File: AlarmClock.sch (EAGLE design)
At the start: 22 parts, among them IC1 LD1117AS33TR, T1 BC817-25LT1SMD

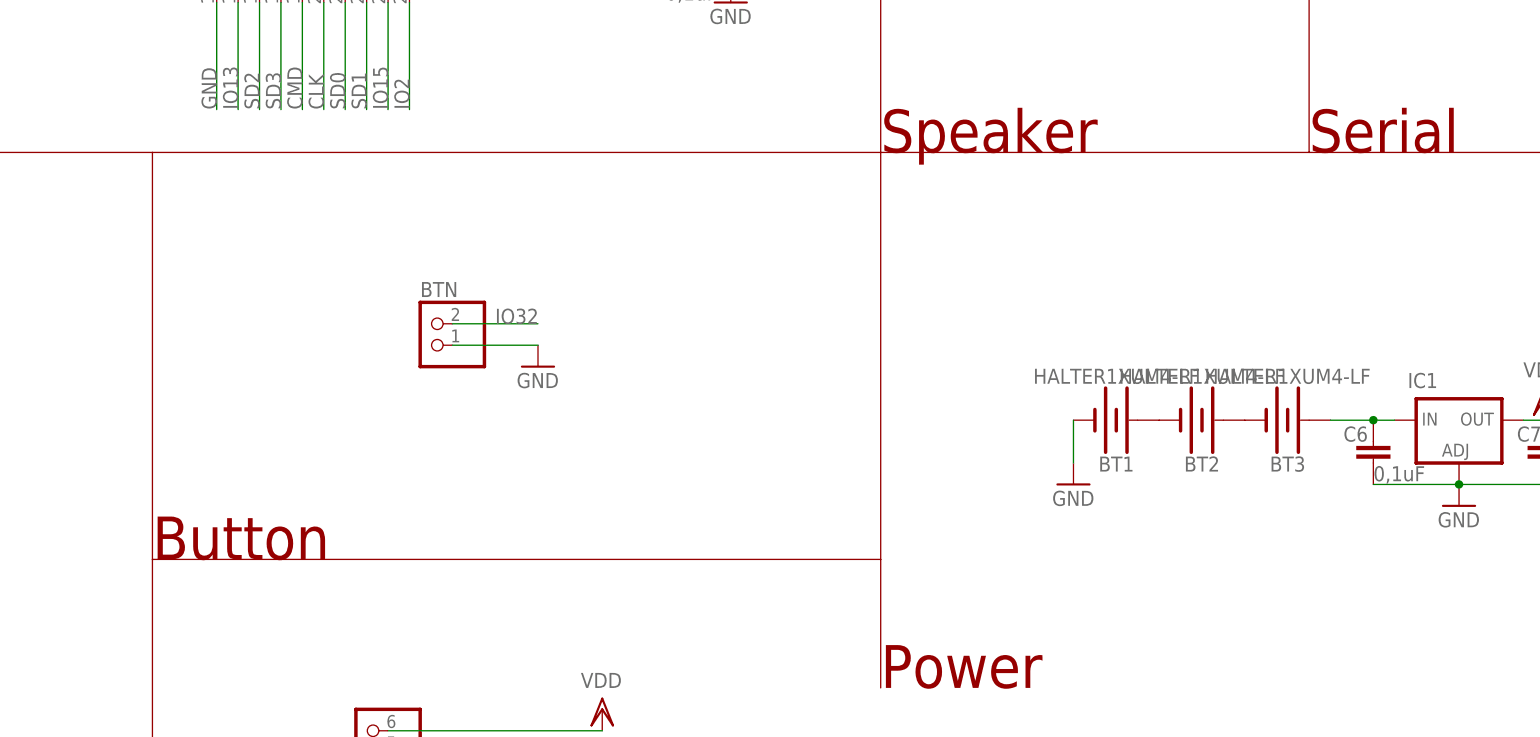
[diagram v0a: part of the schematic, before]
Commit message: Add files via upload
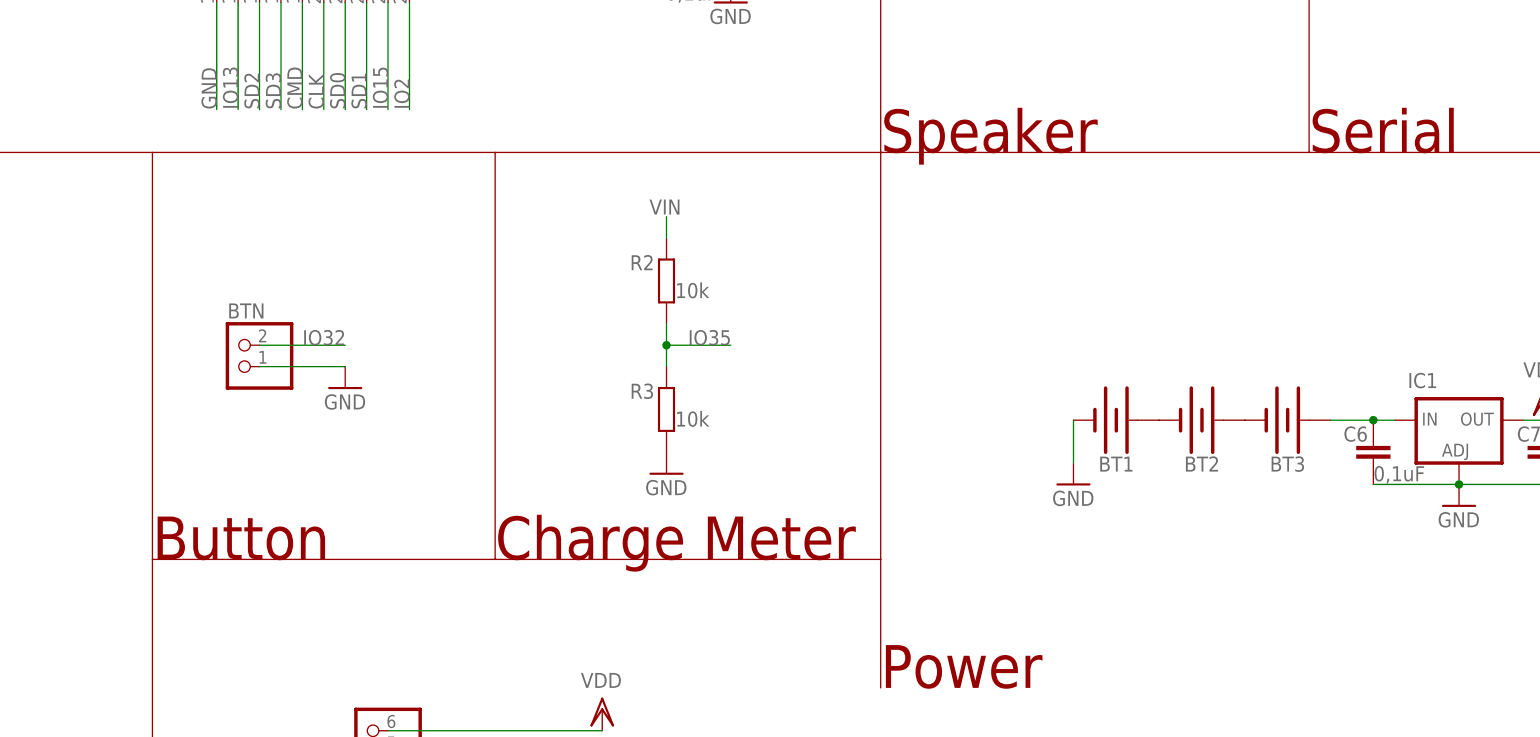
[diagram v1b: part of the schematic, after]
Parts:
- added R2, R3: 10k, rcl:R-EU_R1206
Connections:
- net GND: now also R3.1
- net IO35: now also R2.1, R3.2
- net VIN: now also R2.2
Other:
- note added: "Charge Meter"
- moved on the sheet: BTN
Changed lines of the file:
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@@
 <part name="GND9" library="supply1" library_urn="urn:adsk.eagle:library:371" deviceset="GND" device=""/>
 <part name="RST" library="rcl" library_urn="urn:adsk.eagle:library:334" deviceset="R-EU_" device="R1206" package3d_urn="urn:adsk.eagle:package:23540/2"/>
+<part name="R2" library="rcl" library_urn="urn:adsk.eagle:library:334" deviceset="R-EU_" device="R1206" package3d_urn="urn:adsk.eagle:package:23540/2" value="10k"/>
+<part name="R3" library="rcl" library_urn="urn:adsk.eagle:library:334" deviceset="R-EU_" device="R1206" package3d_urn="urn:adsk.eagle:package:23540/2" value="10k"/>
+<part name="GND10" library="supply1" library_urn="urn:adsk.eagle:library:371" deviceset="GND" device=""/>
 </parts>
 <sheets>
@@
 <text x="162.56" y="35.56" size="5.08" layer="94">Power</text>
 <text x="253.492" y="7.112" size="2.54" layer="94">1.0</text>
-<wire x1="162.56" y1="99.06" x2="76.2" y2="99.06" width="0.1524" layer="94"/>
+<wire x1="162.56" y1="99.06" x2="116.84" y2="99.06" width="0.1524" layer="94"/>
+<wire x1="116.84" y1="99.06" x2="76.2" y2="99.06" width="0.1524" layer="94"/>
 <wire x1="76.2" y1="99.06" x2="0" y2="99.06" width="0.1524" layer="94"/>
 <wire x1="162.56" y1="99.06" x2="162.56" y2="180.34" width="0.1524" layer="94"/>
@@
 <wire x1="76.2" y1="0" x2="76.2" y2="50.8" width="0.1524" layer="94"/>
 <wire x1="76.2" y1="50.8" x2="76.2" y2="99.06" width="0.1524" layer="94"/>
-<wire x1="76.2" y1="50.8" x2="162.56" y2="50.8" width="0.1524" layer="94"/>
+<wire x1="76.2" y1="50.8" x2="116.84" y2="50.8" width="0.1524" layer="94"/>
 <text x="0" y="0" size="5.08" layer="94">LCD</text>
 <text x="76.2" y="0" size="5.08" layer="94">Sensor</text>
@@
 <text x="213.36" y="99.06" size="5.08" layer="94">Serial</text>
 <text x="162.56" y="99.06" size="5.08" layer="94">Speaker</text>
+<wire x1="116.84" y1="50.8" x2="162.56" y2="50.8" width="0.1524" layer="94"/>
 <wire x1="213.36" y1="99.06" x2="213.36" y2="180.34" width="0.1524" layer="94"/>
+<text x="116.84" y="50.8" size="5.08" layer="94">Charge Meter</text>
+<wire x1="116.84" y1="50.8" x2="116.84" y2="99.06" width="0.1524" layer="94"/>
 </plain>
 <instances>
@@
 <instance part="BT3" gate="G$1" x="210.82" y="67.31" smashed="yes" rot="R180">
 <attribute name="NAME" x="210.82" y="62.992" size="1.778" layer="95" font="vector" rot="R180" align="bottom-center"/>
-<attribute name="VALUE" x="210.82" y="71.628" size="1.778" layer="96" font="vector" rot="R180" align="top-center"/>
 </instance>
 <instance part="BT1" gate="G$1" x="190.5" y="67.31" smashed="yes" rot="R180">
 <attribute name="NAME" x="190.5" y="62.992" size="1.778" layer="95" font="vector" rot="R180" align="bottom-center"/>
-<attribute name="VALUE" x="190.5" y="71.628" size="1.778" layer="96" font="vector" rot="R180" align="top-center"/>
 </instance>
 <instance part="GND14" gate="1" x="185.42" y="59.69" smashed="yes">
@@
 <instance part="BT2" gate="G$1" x="200.66" y="67.31" smashed="yes" rot="R180">
 <attribute name="NAME" x="200.66" y="62.992" size="1.778" layer="95" font="vector" rot="R180" align="bottom-center"/>
-<attribute name="VALUE" x="200.66" y="71.628" size="1.778" layer="96" font="vector" rot="R180" align="top-center"/>
 </instance>
 <instance part="BOOT" gate="G$1" x="137.16" y="127" smashed="yes">
@@
 <attribute name="VALUE" x="195.58" y="160.02" size="1.778" layer="96"/>
 </instance>
-<instance part="GND5" gate="1" x="121.92" y="73.66" smashed="yes">
-<attribute name="VALUE" x="119.38" y="71.12" size="1.778" layer="96"/>
-</instance>
-<instance part="BTN" gate="G$1" x="109.22" y="78.74" smashed="yes" rot="R180">
-<attribute name="NAME" x="107.95" y="81.915" size="1.778" layer="95"/>
-<attribute name="VALUE" x="115.57" y="83.82" size="1.778" layer="96" rot="R180"/>
+<instance part="GND5" gate="1" x="99.06" y="71.12" smashed="yes">
+<attribute name="VALUE" x="96.52" y="68.58" size="1.778" layer="96"/>
+</instance>
+<instance part="BTN" gate="G$1" x="86.36" y="76.2" smashed="yes" rot="R180">
+<attribute name="NAME" x="85.09" y="79.375" size="1.778" layer="95"/>
+<attribute name="VALUE" x="92.71" y="81.28" size="1.778" layer="96" rot="R180"/>
 </instance>
 <instance part="VDD6" gate="G$1" x="53.34" y="27.94" smashed="yes">
@@
 <attribute name="NAME" x="10.3886" y="156.21" size="1.778" layer="95"/>
 <attribute name="VALUE" x="10.668" y="153.924" size="1.778" layer="96" rot="R270"/>
+</instance>
+<instance part="R2" gate="G$1" x="137.16" y="83.82" smashed="yes" rot="R90">
+<attribute name="NAME" x="132.8166" y="85.09" size="1.778" layer="95"/>
+<attribute name="VALUE" x="138.176" y="81.788" size="1.778" layer="96"/>
+</instance>
+<instance part="R3" gate="G$1" x="137.16" y="68.58" smashed="yes" rot="R90">
+<attribute name="NAME" x="132.8166" y="69.85" size="1.778" layer="95"/>
+<attribute name="VALUE" x="138.176" y="66.548" size="1.778" layer="96"/>
+</instance>
+<instance part="GND10" gate="1" x="137.16" y="60.96" smashed="yes">
+<attribute name="VALUE" x="134.62" y="58.42" size="1.778" layer="96"/>
 </instance>
 </instances>
@@
 <pinref part="BTN" gate="G$1" pin="1"/>
 <pinref part="GND5" gate="1" pin="GND"/>
-<wire x1="121.92" y1="76.2" x2="111.76" y2="76.2" width="0.1524" layer="91"/>
+<wire x1="99.06" y1="73.66" x2="88.9" y2="73.66" width="0.1524" layer="91"/>
 </segment>
 <segment>
@@
 <junction x="7.62" y="147.32"/>
 <pinref part="RST" gate="G$1" pin="1"/>
+</segment>
+<segment>
+<pinref part="GND10" gate="1" pin="GND"/>
+<pinref part="R3" gate="G$1" pin="1"/>
 </segment>
 </net>
@@
 <label x="55.88" y="144.78" size="1.778" layer="95"/>
 </segment>
+<segment>
+<pinref part="R3" gate="G$1" pin="2"/>
+<pinref part="R2" gate="G$1" pin="1"/>
+<wire x1="137.16" y1="73.66" x2="137.16" y2="76.2" width="0.1524" layer="91"/>
+<wire x1="137.16" y1="76.2" x2="137.16" y2="78.74" width="0.1524" layer="91"/>
+<wire x1="137.16" y1="76.2" x2="144.78" y2="76.2" width="0.1524" layer="91"/>
+<junction x="137.16" y="76.2"/>
+<label x="139.7" y="76.2" size="1.778" layer="95"/>
+</segment>
 </net>
 <net name="IO26" class="0">
@@
 <label x="231.14" y="132.08" size="1.778" layer="95"/>
 </segment>
+<segment>
+<pinref part="R2" gate="G$1" pin="2"/>
+<wire x1="137.16" y1="88.9" x2="137.16" y2="91.44" width="0.1524" layer="91"/>
+<label x="135.128" y="91.694" size="1.778" layer="95"/>
+</segment>
 </net>
 <net name="IO32" class="0">
@@
 <segment>
 <pinref part="BTN" gate="G$1" pin="2"/>
-<wire x1="111.76" y1="78.74" x2="121.92" y2="78.74" width="0.1524" layer="91"/>
-<label x="116.84" y="78.74" size="1.778" layer="95"/>
-</segment>
-</net>
+<wire x1="88.9" y1="76.2" x2="99.06" y2="76.2" width="0.1524" layer="91"/>
+<label x="93.98" y="76.2" size="1.778" layer="95"/>
+</segment>
+</net>
